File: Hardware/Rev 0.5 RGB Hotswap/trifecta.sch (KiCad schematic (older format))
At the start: 280 parts, among them J1 USB2_C_Receptacle, SW1 RESET, SW2 Rotary_Encoder_Switch, SW3 Rotary_Encoder_Switch, SW4 Rotary_Encoder_Switch, U1 ATmega32U4-AU, U2 SRV05-4, Y1 16MHz

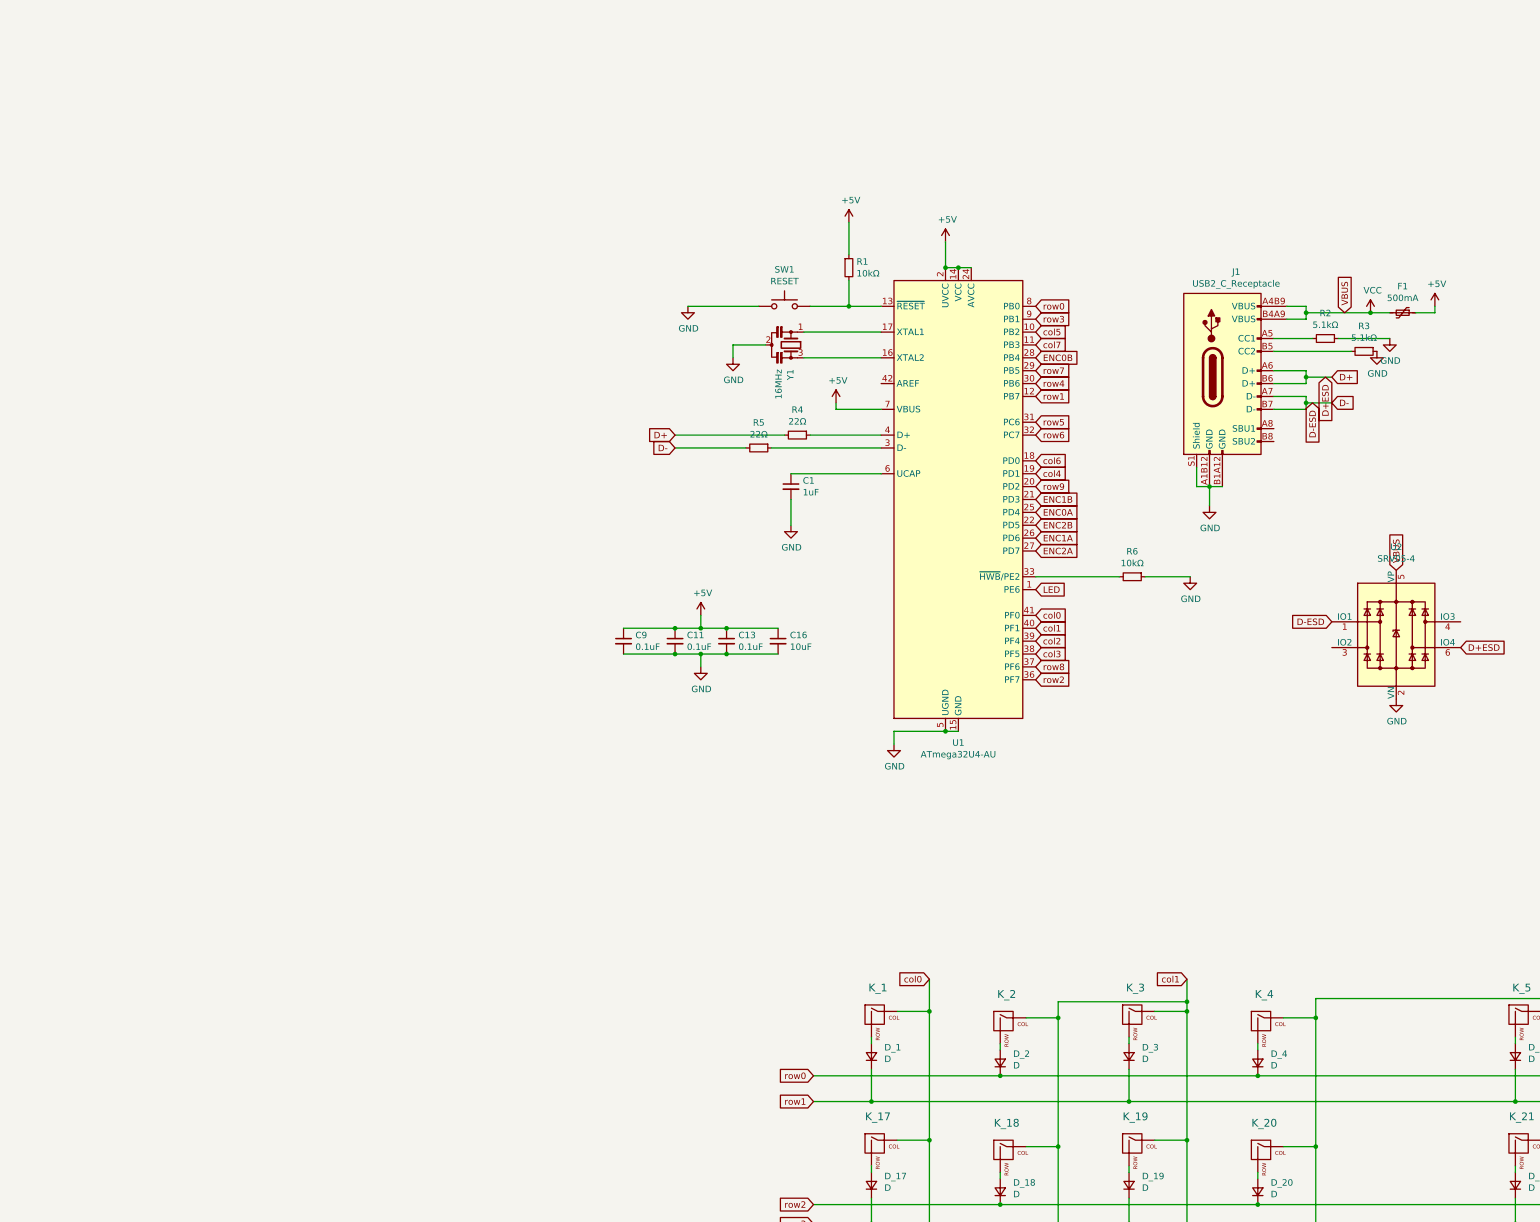
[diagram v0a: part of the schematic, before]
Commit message: 8/8
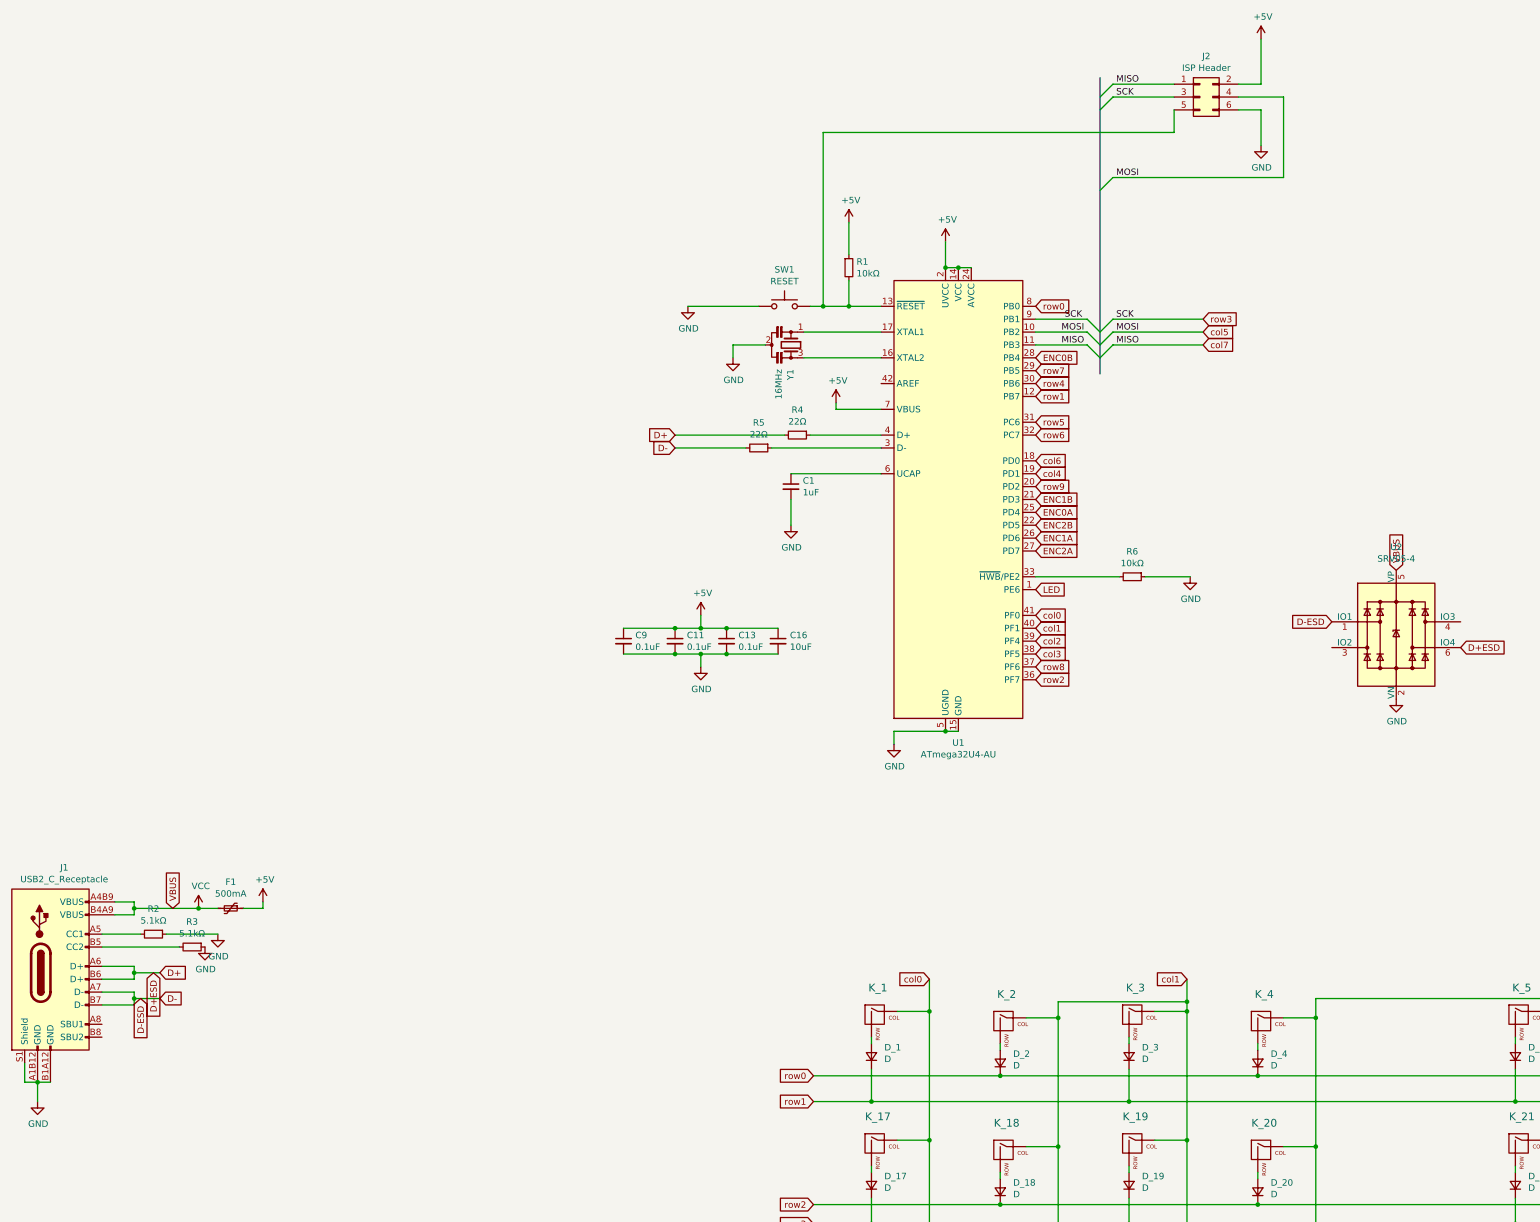
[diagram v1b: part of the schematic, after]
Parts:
- added J2: ISP Header, Connector_PinHeader_2.54mm:PinHeader_2x03_P2.54mm_Vertical, symbol conn:Conn_02x03_Odd_Even
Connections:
- net +5V: now also J2.2 (Pin_2)
- net 0col: now also J2.1 (Pin_1)
- net GND: now also J2.6 (Pin_6)
- net col5: now also J2.4 (Pin_4)
- net row3: now also J2.3 (Pin_3)
- net at R1.2, SW1.2, U1.13 (~RESET): now also J2.5 (Pin_5)
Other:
- moved on the sheet: F1, J1, R2, R3

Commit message: 8/10
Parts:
- F1: LCSC Part# (none) -> C70068; Mfr (none) -> TECHFUSE; Part# (none) -> nSMD025
- R4, R5: LCSC Part# C17560 -> C17561; Part# 0805W8F2202T5E -> 0805W8F220JT5E
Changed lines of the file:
@@
 F 1 "22Ω" V 3245 4100 50  0000 C CNN
 F 2 "Resistor_SMD:R_0805_2012Metric" H 3350 4100 50  0001 C CNN
-F 3 "https://datasheet.lcsc.com/szlcsc/Uniroyal-Elec-0805W8F2202T5E_C17560.pdf" H 3350 4100 50  0001 C CNN
-F 4 "C17560" V 3350 4100 50  0001 C CNN "LCSC Part#"
-F 5 "0805W8F2202T5E" V 3350 4100 50  0001 C CNN "Part#"
+F 3 "https://datasheet.lcsc.com/szlcsc/Uniroyal-Elec-0805W8F220JT5E_C17561.pdf" H 3350 4100 50  0001 C CNN
+F 4 "C17561" V 3350 4100 50  0001 C CNN "LCSC Part#"
+F 5 "0805W8F220JT5E" V 3350 4100 50  0001 C CNN "Part#"
 F 6 "Uniroyal Elec" V 3350 4100 50  0001 C CNN "Mrf"
 	1    3350 4100
@@
 F 1 "22Ω" V 3545 4000 50  0000 C CNN
 F 2 "Resistor_SMD:R_0805_2012Metric" H 3650 4000 50  0001 C CNN
-F 3 "https://datasheet.lcsc.com/szlcsc/Uniroyal-Elec-0805W8F2202T5E_C17560.pdf" H 3650 4000 50  0001 C CNN
-F 4 "C17560" V 3650 4000 50  0001 C CNN "LCSC Part#"
-F 5 "0805W8F2202T5E" V 3650 4000 50  0001 C CNN "Part#"
+F 3 "https://datasheet.lcsc.com/szlcsc/Uniroyal-Elec-0805W8F220JT5E_C17561.pdf" H 3650 4000 50  0001 C CNN
+F 4 "C17561" V 3650 4000 50  0001 C CNN "LCSC Part#"
+F 5 "0805W8F220JT5E" V 3650 4000 50  0001 C CNN "Part#"
 F 6 "Uniroyal Elec" V 3650 4000 50  0001 C CNN "Mrf"
 	1    3650 4000
@@
 F 1 "500mA" V -864 7675 50  0000 C CNN
 F 2 "Fuse:Fuse_1206_3216Metric" H -700 7475 50  0001 L CNN
-F 3 "~" H -750 7675 50  0001 C CNN
-F 4 "" V -750 7675 50  0001 C CNN "LCSC Part#"
-F 5 "" V -750 7675 50  0001 C CNN "Part#"
-F 6 "" V -750 7675 50  0001 C CNN "Mfr"
+F 3 "https://datasheet.lcsc.com/szlcsc/TECHFUSE-nSMD025_C70068.pdf" H -750 7675 50  0001 C CNN
+F 4 "C70068" V -750 7675 50  0001 C CNN "LCSC Part#"
+F 5 "nSMD025" V -750 7675 50  0001 C CNN "Part#"
+F 6 "TECHFUSE" V -750 7675 50  0001 C CNN "Mfr"
 	1    -750 7675
 	0    1    1    0
@@
 Wire Wire Line
 	6100 3300 6800 3300
-Wire Bus Line
-	6000 1225 6000 3525
 Text Label 5725 3100 0    50   ~ 0
 SCK
@@
 Text Label 6125 3300 0    50   ~ 0
 MISO
+Wire Bus Line
+	6000 1225 6000 3525
 $EndSCHEMATC
